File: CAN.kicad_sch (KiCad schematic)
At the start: 9 parts, among them U4 TCAN337, U5 CDSOT23-T24CAN

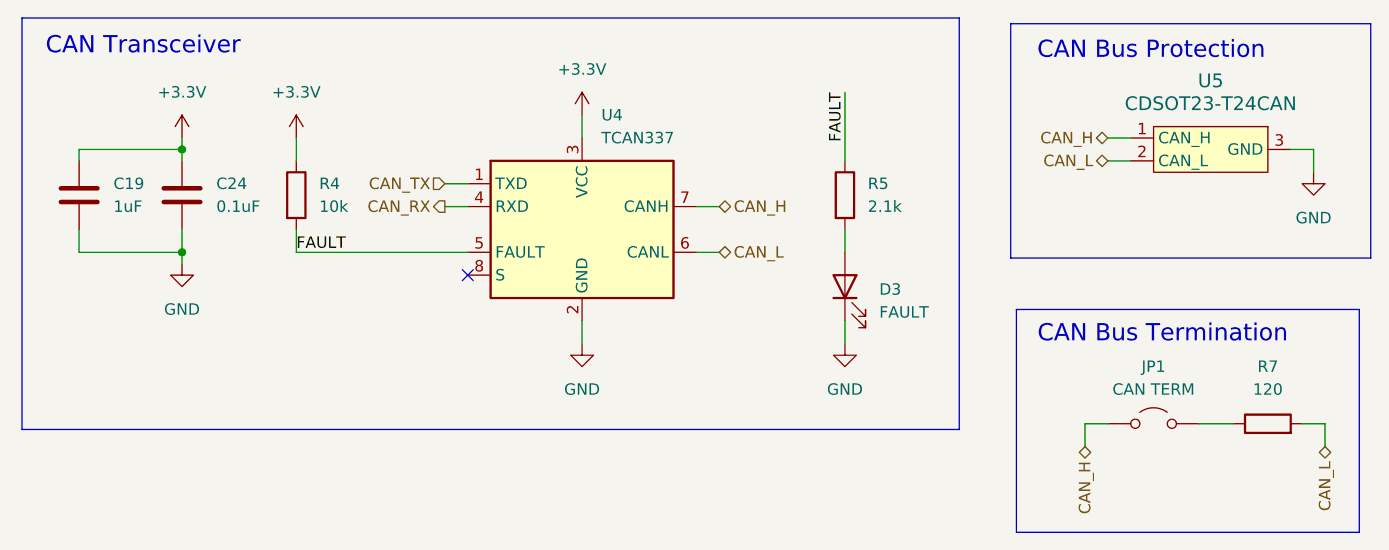
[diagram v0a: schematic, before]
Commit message: finish mcu breakouts
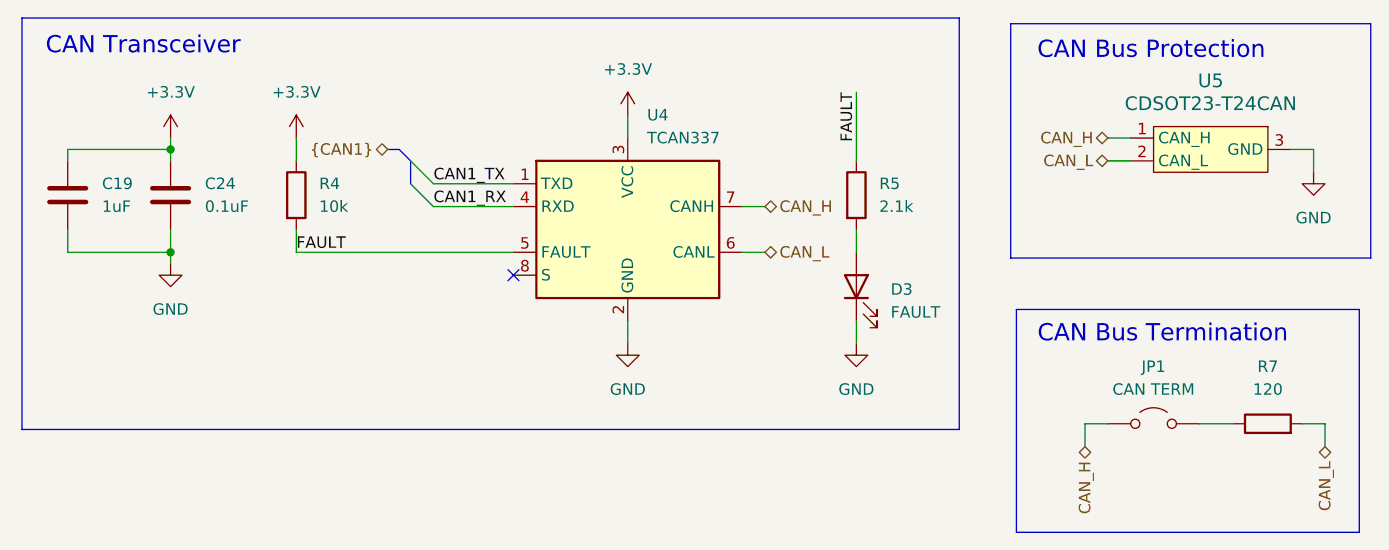
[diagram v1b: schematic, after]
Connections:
- net CAN_RX renamed CAN1_RX
- net CAN_TX renamed CAN1_TX
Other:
- moved on the sheet: C19, C24, D3, R5, U4
